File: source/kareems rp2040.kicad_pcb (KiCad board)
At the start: 2 copper layers, 29 x 57 mm, 37 parts, among them J1 USB_C_Receptacle_USB2.0_14P, J2 Conn_01x20, J3 Conn_01x20, J4 Conn_01x03, SW1 SW_Push, U1 RP2040, U2 W25Q16JVSS, U4 MCP1700x-330xxTT, Y1 12MHz

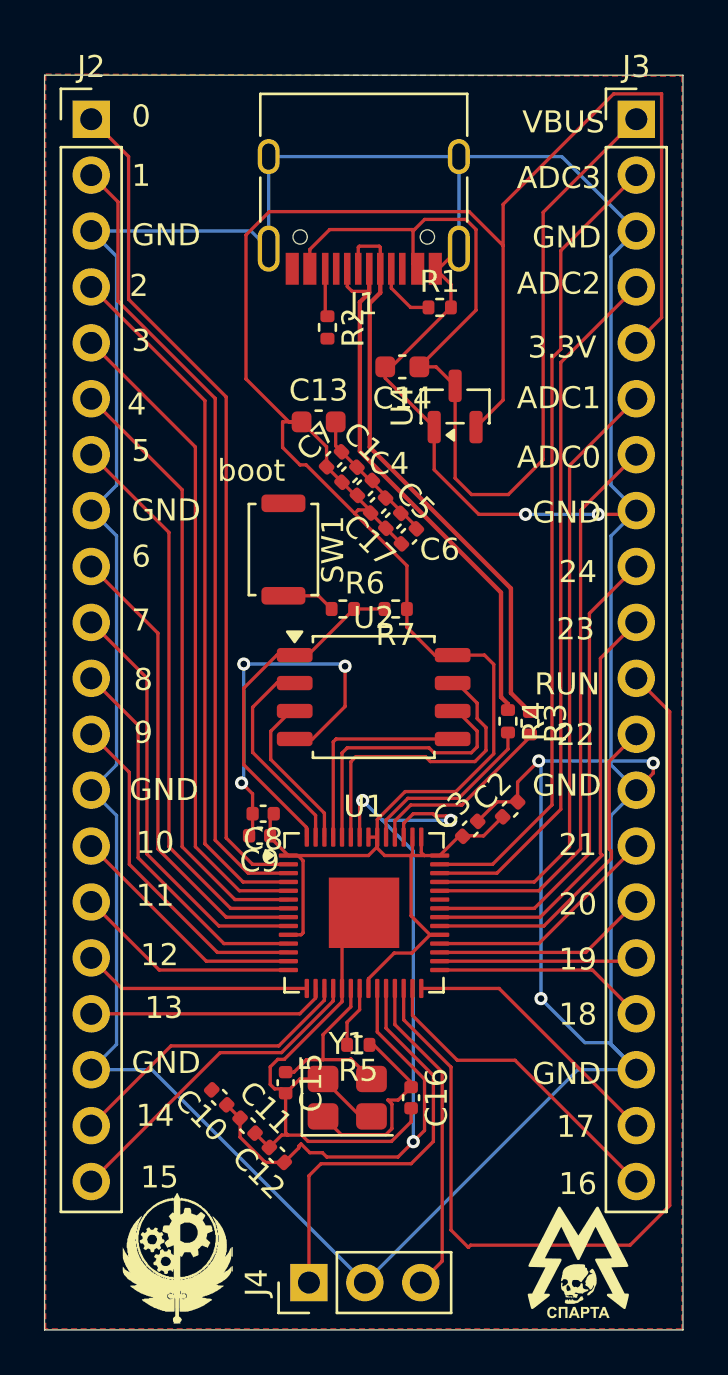
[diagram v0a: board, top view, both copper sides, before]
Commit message: e
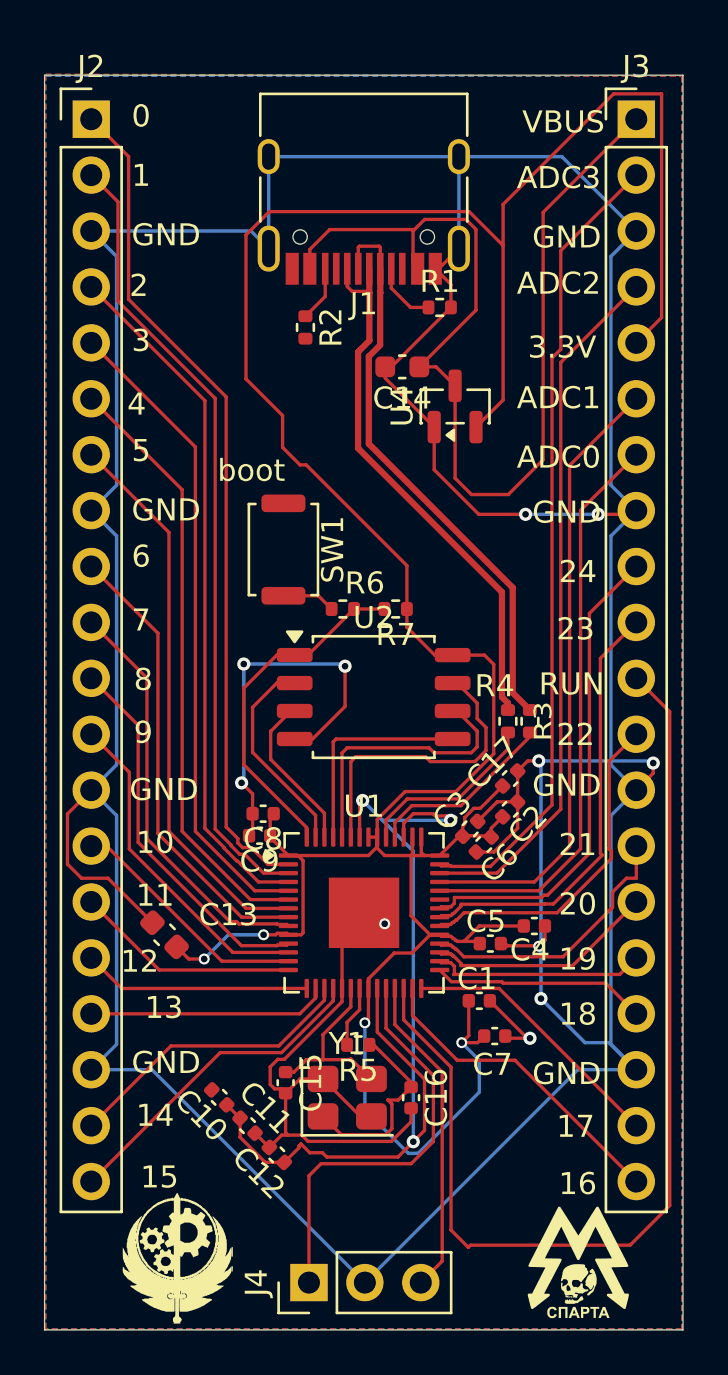
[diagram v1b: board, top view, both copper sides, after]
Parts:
- added G***: LOGO, drawings:heart, B.Cu at (205.2, 99.0)
- moved C7 27.2 mm to (219.2, 108.9), turned to 0 degrees
- moved C1 24.6 mm to (218.5, 107.3), turned to 0 degrees
- moved C13 24.3 mm to (204.2, 104.3), turned to 135 degrees
- moved C4 21.3 mm to (221.0, 103.9), turned to 0 degrees
- moved C5 19.7 mm to (219.0, 104.7), turned to 0 degrees
- moved C6 14.4 mm to (218.7, 100.2), turned to -135 degrees
- moved C17 13.8 mm to (219.9, 97.2)
- moved R2 1.00 mm to (210.6, 76.7)
- moved R3 0.09 mm to (220.8, 94.6)
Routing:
- net +3.3V: track 121.1 -> 144.0 mm, vias 0 -> 4
- net GND: track 250.5 -> 263.3 mm, vias 8 -> 11
- net GPIO21: track 10.8 -> 12.5 mm
- net GPIO19: track 8.99 -> 9.75 mm
- net GPIO20: track 9.88 -> 10.4 mm
- added copper zone on B.Cu, net GND
